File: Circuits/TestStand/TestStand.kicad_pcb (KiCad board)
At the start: 2 copper layers, 105 x 142.5 mm, 109 parts, among them IC1 STP85NF55, J1 2601-1107, J10 Screw_Terminal_01x03, J11 Screw_Terminal_01x03, J12 Screw_Terminal_01x03, J13 Screw_Terminal_01x03, J14 CONN4_2606-1104/010-000_WAG, J15 Conn_Coaxial, J18 2601-1107, J2 2601-1107, J3 Screw_Terminal_01x03, J4 Screw_Terminal_01x03, J5 Screw_Terminal_01x03, J6 Screw_Terminal_01x03, J7 Screw_Terminal_01x03, J8 Screw_Terminal_01x03, J9 Screw_Terminal_01x03, Q1 MMBT4403-7-F, Q2 MMBT4403-7-F, Q3 MMBT4403-7-F, U1 HX711, U2 HX711, U3 HX711, U4 Teensy4.1, U5 LP2980IM5X-3.3/NOPB, U6 MAX31855KASA, U7 NRF24L01, U8 LP2980IM5X-3.3/NOPB, Y1 16Mhz

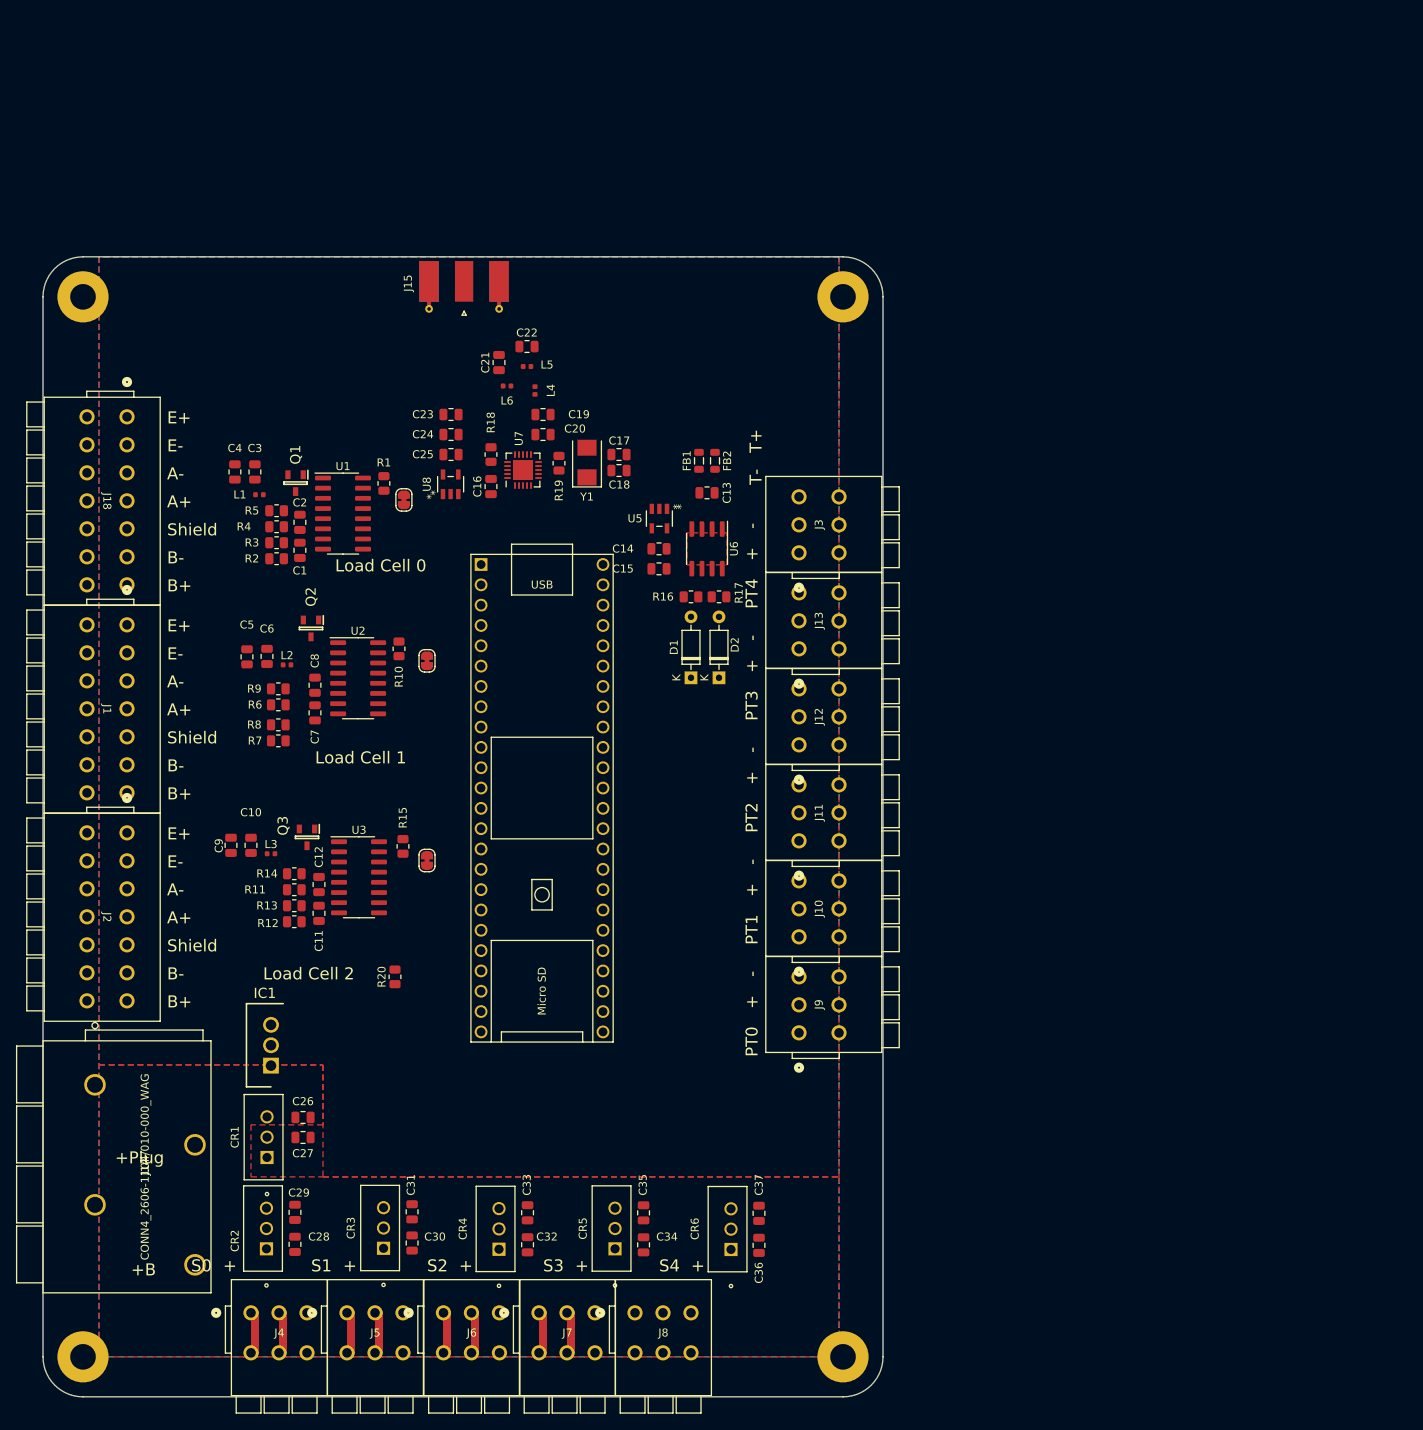
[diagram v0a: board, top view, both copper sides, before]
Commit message: help
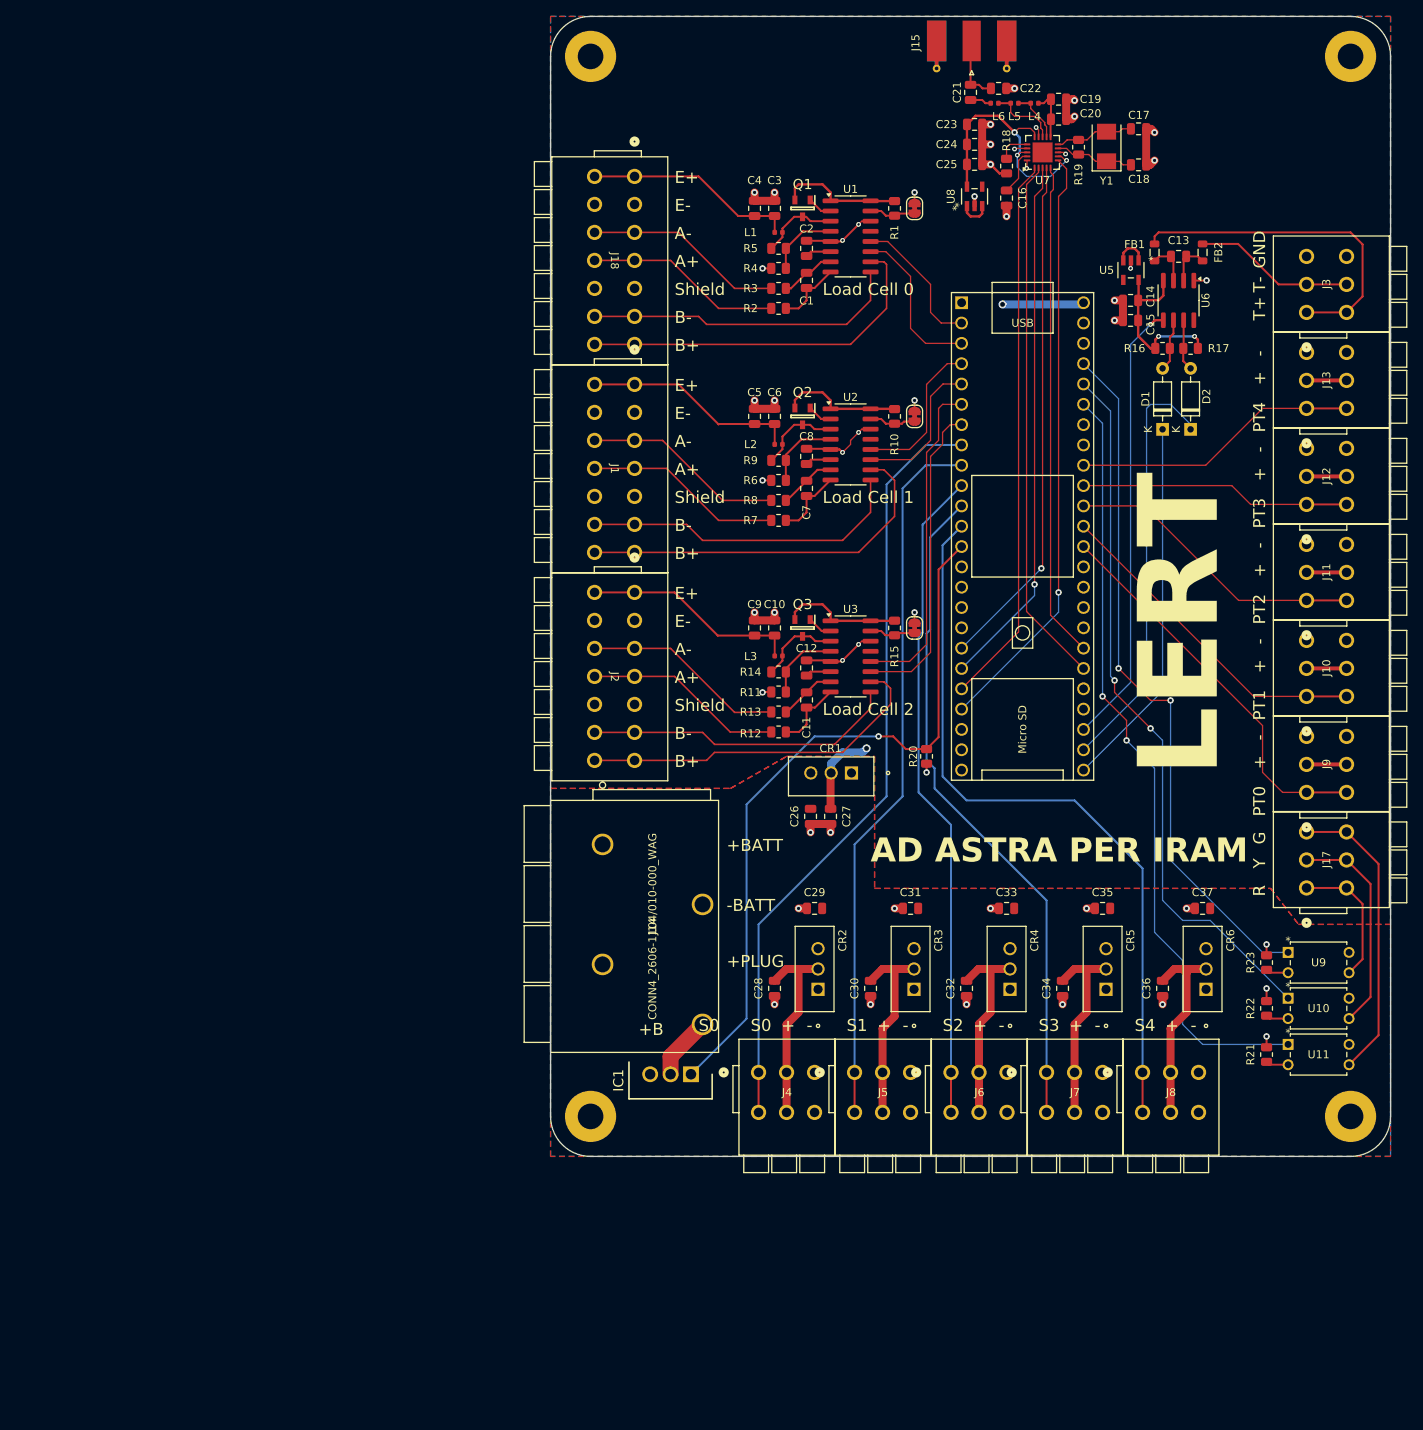
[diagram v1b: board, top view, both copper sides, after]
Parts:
- added J17: Screw_Terminal_01x03, Library:CONN3_2601-1103_WAG, F.Cu at (173.4, 141.9)
- added R21: 220, Resistor_SMD:R_0805_2012Metric, F.Cu at (168.4, 162.7)
- added R22: 220, Resistor_SMD:R_0805_2012Metric, F.Cu at (168.4, 156.9)
- added R23: 220, Resistor_SMD:R_0805_2012Metric, F.Cu at (168.4, 151.2)
- added U10: VO615A-X001, Library:DIP-4_VO615A_VIS, F.Cu at (171.1, 155.7)
- added U11: VO615A-X001, Library:DIP-4_VO615A_VIS, F.Cu at (171.1, 161.4)
- added U9: VO615A-X001, Library:DIP-4_VO615A_VIS, F.Cu at (171.1, 149.9)
- moved CR1 87.5 mm to (116.6, 127.5), turned to 180 degrees
- moved C27 77.2 mm to (113.9, 132.9), turned to 90 degrees
- moved C17 76.6 mm to (152.4, 47.0)
- moved CR2 76.2 mm to (112.4, 154.6)
- moved U7 76.1 mm to (140.4, 49.9)
- moved R19 76.0 mm to (144.9, 49.3)
- moved Y1 76.0 mm to (148.4, 49.2)
- moved C19 75.5 mm to (142.4, 43.3)
- moved C20 75.5 mm to (142.4, 45.8)
- moved C18 75.4 mm to (152.4, 51.5)
- moved C29 75.2 mm to (111.9, 144.4), turned to 0 degrees
- moved C23 74.8 mm to (131.9, 46.4)
- moved C24 74.8 mm to (131.9, 48.9)
- moved C25 74.8 mm to (131.9, 51.4)
- moved U8 74.7 mm to (131.9, 55.4)
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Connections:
- J3 pad 5: unconnected-(J3-3_1-Pad5) -> GND
- J3 pad 6: unconnected-(J3-3_2-Pad6) -> GND
- U4 pad 43: unconnected-(U4-21_A7_RX5_BCLK1-Pad43) -> /GPIN
- U4 pad 44: unconnected-(U4-22_A8_CTX1-Pad44) -> /YPIN
- U4 pad 45: unconnected-(U4-23_A9_CRX1_MCLK1-Pad45) -> /RPIN
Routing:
- net GND: track 0.00 -> 107.6 mm, vias 0 -> 52
- net +5V: track 0.00 -> 100.6 mm, vias 0 -> 2
- net /GPIN: track 0.00 -> 96.9 mm, vias 0 -> 2
- net /PWM4: track 0.00 -> 92.5 mm
- net /PWM0: track 5.00 -> 96.5 mm
- net /GP: track 0.00 -> 90.4 mm, vias 0 -> 1
- net /YPIN: track 0.00 -> 89.4 mm, vias 0 -> 2
- net /RPIN: track 0.00 -> 87.5 mm, vias 0 -> 2
- net /PWM1: track 5.00 -> 89.1 mm
- net /PWM3: track 5.00 -> 83.8 mm
- net /PWM2: track 5.00 -> 82.3 mm
- net /rIRQ: track 0.00 -> 74.5 mm, vias 0 -> 1
- net /rCE: track 0.00 -> 68.9 mm
- net /rSCK: track 0.00 -> 66.8 mm, vias 0 -> 1
- net /rCSN: track 0.00 -> 66.1 mm
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- removed copper zone on F.Cu, net GND
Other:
- board text added: "+BATT"
- board text added: "+PLUG"
- board text added: "-BATT"
- board text added: "AD ASTRA PER IRAM"
- board text added: "G"
- board text added: "GND"
- board text added: "LERT"
- board text added: "R"
- board text added: "V0.1 PCB By Isaac Sal"
- board text added: "Y"
- board text removed: "+Plug"
